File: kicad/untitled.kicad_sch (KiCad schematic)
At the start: 22 parts, among them SW1 SW_SPDT, SW11 SW_Push_SPDT, SW12 SW_Push_SPDT, SW13 SW_Push_SPDT, SW14 SW_Push_SPDT, SW15 SW_Push_SPDT, SW16 SW_Push_SPDT, SW17 SW_Push_SPDT, SW18 SW_Push_SPDT, SW2 SW_SPDT, SW3 SW_SPDT, SW4 SW_SPDT, SW5 SW_SPDT

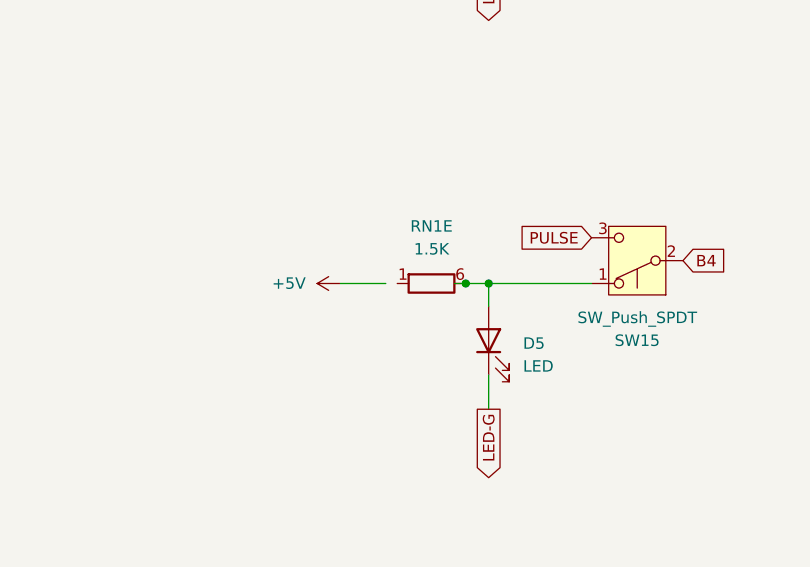
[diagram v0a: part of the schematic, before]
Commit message: Starting docs
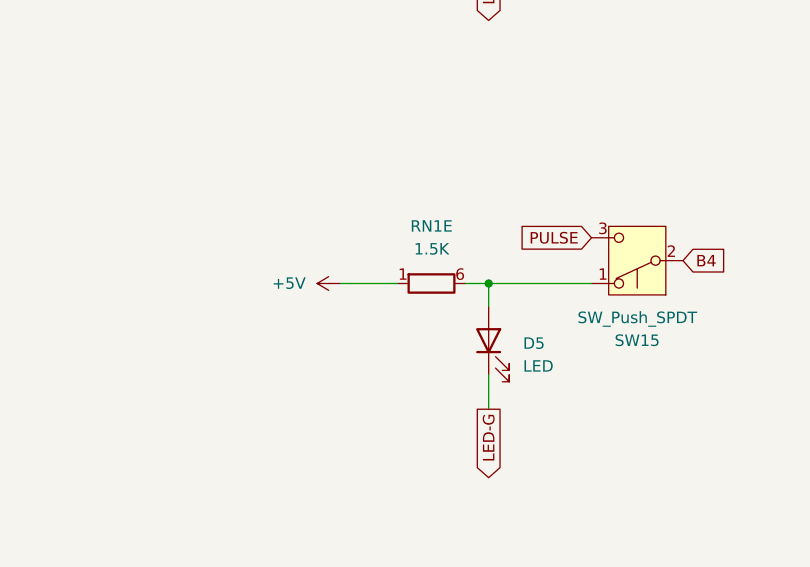
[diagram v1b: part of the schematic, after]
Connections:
- net +5V: now also RN1.1 (R1)
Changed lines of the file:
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@@
 (kicad_sch
-	(version 20231120)
+	(version 20250114)
 	(generator "eeschema")
-	(generator_version "8.0")
+	(generator_version "9.0")
 	(paper "A3")
 	(title_block
 		(title "PROM Programmer")
-		(date "2024-11-17")
-		(rev "V1.1")
+		(date "2025-03-27")
+		(rev "V1.4")
 	)
-	(junction
-		(at 140.97 167.64)
-		(diameter 0)
-		(color 0 0 0 0)
+	(text "800USP8P1A1M2RE"
+		(exclude_from_sim no)
+		(at 144.78 45.212 0)
+		(effects
+			(font
+				(size 2.54 2.54)
+				(thickness 0.254)
+				(bold yes)
+			)
+		)
+	)
+	(text "GW12LCP"
+		(exclude_from_sim no)
+		(at 64.008 46.482 0)
+		(effects
+			(font
+				(size 2.54 2.54)
+				(thickness 0.254)
+				(bold yes)
+			)
+		)
 	)
 	(junction
@@
 	)
 	(junction
-		(at 207.01 116.84)
+		(at 143.51 167.64)
 		(diameter 0)
 		(color 0 0 0 0)
 	)
 	(junction
-		(at 207.01 167.64)
+		(at 207.01 116.84)
 		(diameter 0)
 		(color 0 0 0 0)
 	)
 	(junction
-		(at 207.01 66.04)
+		(at 207.01 167.64)
 		(diameter 0)
 		(color 0 0 0 0)
 	)
 	(junction
-		(at 143.51 167.64)
+		(at 207.01 66.04)
 		(diameter 0)
 		(color 0 0 0 0)
@@
 	(wire
 		(pts
-			(xy 140.97 167.64) (xy 143.51 167.64)
-		)
-		(stroke
-			(width 0)
-			(type default)
-		)
-	)
-	(wire
-		(pts
 			(xy 38.1 167.64) (xy 50.8 167.64)
 		)
@@
 	(wire
 		(pts
+			(xy 140.97 167.64) (xy 143.51 167.64)
+		)
+		(stroke
+			(width 0)
+			(type default)
+		)
+	)
+	(wire
+		(pts
 			(xy 38.1 116.84) (xy 38.1 142.24)
 		)
@@
 	(wire
 		(pts
-			(xy 139.7 167.64) (xy 140.97 167.64)
-		)
-		(stroke
-			(width 0)
-			(type default)
-		)
-	)
-	(wire
-		(pts
 			(xy 207.01 218.44) (xy 218.44 218.44)
 		)
@@
 	(wire
 		(pts
-			(xy 127 167.64) (xy 132.08 167.64)
+			(xy 127 167.64) (xy 133.35 167.64)
 		)
 		(stroke
@@
 		)
 	)
-	(text "800USP8P1A1M2RE"
-		(exclude_from_sim no)
-		(at 144.78 45.212 0)
-		(effects
-			(font
-				(size 2.54 2.54)
-				(thickness 0.254)
-				(bold yes)
-			)
-		)
-	)
-	(text "GW12LCP"
-		(exclude_from_sim no)
-		(at 64.008 46.482 0)
-		(effects
-			(font
-				(size 2.54 2.54)
-				(thickness 0.254)
-				(bold yes)
-			)
-		)
-	)
 	(global_label "LED-G"
 		(shape output)
@@
 			)
 		)
+		(property "Sim.Pins" "1=K 2=A"
+			(at 143.51 173.99 0)
+			(effects
+				(font
+					(size 1.27 1.27)
+				)
+				(hide yes)
+			)
+		)
 		(pin "2"
 		)
@@
 			)
 		)
+		(property "Sim.Pins" "1=K 2=A"
+			(at 143.51 123.19 0)
+			(effects
+				(font
+					(size 1.27 1.27)
+				)
+				(hide yes)
+			)
+		)
 		(pin "2"
 		)
@@
 			)
 		)
+		(property "Sim.Pins" "1=K 2=A"
+			(at 143.51 72.39 0)
+			(effects
+				(font
+					(size 1.27 1.27)
+				)
+				(hide yes)
+			)
+		)
 		(pin "2"
 		)
@@
 			)
 		)
+		(property "Sim.Pins" "1=K 2=A"
+			(at 207.01 224.79 0)
+			(effects
+				(font
+					(size 1.27 1.27)
+				)
+				(hide yes)
+			)
+		)
 		(pin "2"
 		)
@@
 			)
 		)
+		(property "Sim.Pins" "1=K 2=A"
+			(at 143.51 224.79 0)
+			(effects
+				(font
+					(size 1.27 1.27)
+				)
+				(hide yes)
+			)
+		)
 		(pin "2"
 		)
@@
 			)
 		)
+		(property "Sim.Pins" "1=K 2=A"
+			(at 207.01 123.19 0)
+			(effects
+				(font
+					(size 1.27 1.27)
+				)
+				(hide yes)
+			)
+		)
 		(pin "2"
 		)
@@
 			)
 		)
+		(property "Sim.Pins" "1=K 2=A"
+			(at 207.01 72.39 0)
+			(effects
+				(font
+					(size 1.27 1.27)
+				)
+				(hide yes)
+			)
+		)
 		(pin "2"
 		)
@@
 			(at 207.01 173.99 0)
 			(effects
+				(font
+					(size 1.27 1.27)
+				)
+				(hide yes)
+			)
+		)
+		(property "Sim.Pins" "1=K 2=A"
+			(at 207.01 173.99 0)
+			(effects
